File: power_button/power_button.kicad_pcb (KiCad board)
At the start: 2 copper layers, 24 x 20 mm, 4 parts, among them J1 PWR_KEY, SW1 K6-6277D-02

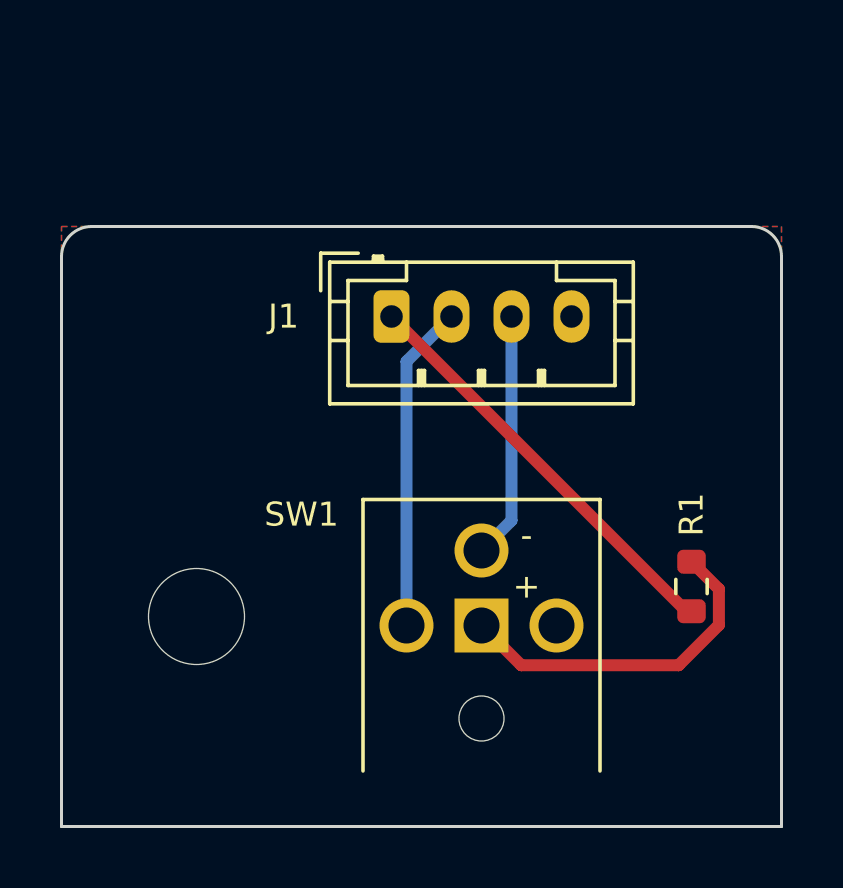
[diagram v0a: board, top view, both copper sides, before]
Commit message: Route the pcb
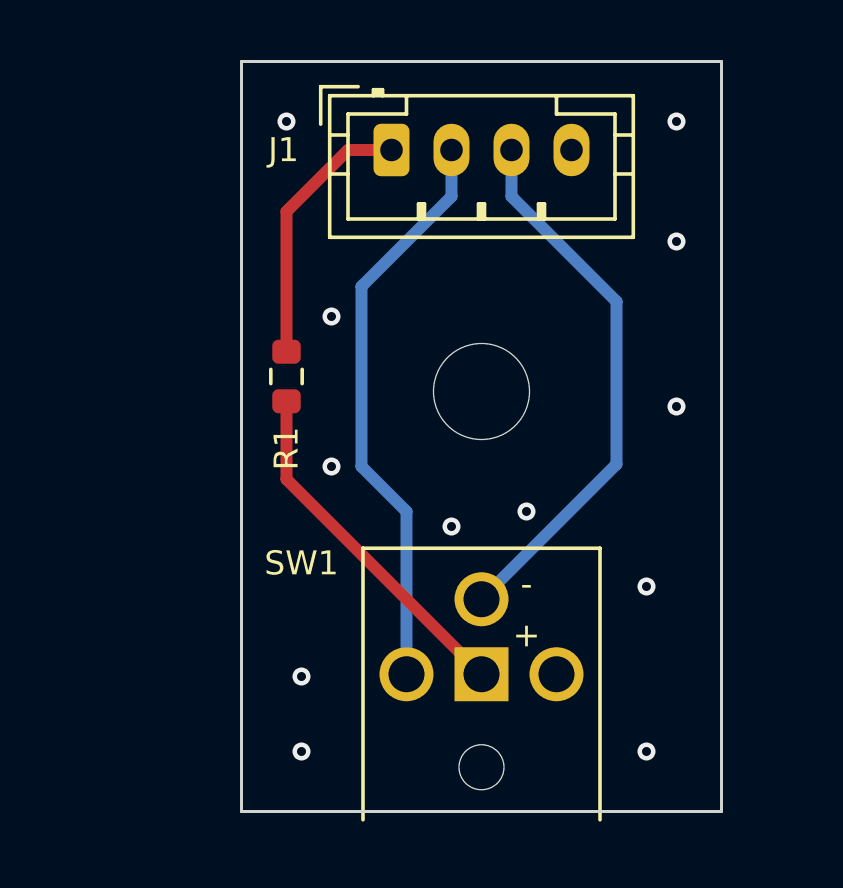
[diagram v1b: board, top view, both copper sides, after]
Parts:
- moved R1 15.2 mm to (107.5, 105.0), turned to -90 degrees
- moved H1 12.1 mm to (114.0, 105.5)
- moved J1 5.55 mm to (111.0, 97.5)
- moved SW1 1.62 mm to (114.0, 114.9)
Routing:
- net /LED_CTRL: track 8.21 -> 18.3 mm
- net /SW: track 10.9 -> 19.3 mm
- net +5V: track 14.1 -> 9.02 mm
- net GND: vias 0 -> 12
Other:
- board size 24 x 20 mm -> 16 x 25 mm
